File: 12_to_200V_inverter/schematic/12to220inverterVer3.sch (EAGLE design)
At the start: 246 parts, among them IC1 UC3842, IC10 TL494, IC2 PC817, IC3 LM358SOIC8, IC4 TL431, IC5 LM317, IC6 74HC595, IC7 74HC595, IC8 ATTINY45, T1 AO4407AL, T10 16N60, T11 BC847, T12 BC847, T13 BSS84, T14 BC857, T15 BC847, T16 BSS84, T17 BC847, T18 BC847, T19 BSS84, T2 IRF830, T20 BSS84, T21 BC847, T22 BC847, T23 BSS84, T24 BC847, T3 IRF830, T4 BC847, T5 BC857, T6 BC857, T7 IRFZ24N, T8 IRFZ24N, T9 BC857, X1 BAT+, X2 LAMP1, X3 LAMP1, X4 BAT-, X5 220VAC, X6 LAMP1_SWITCH, X7 LAMP1_SWITCH, X8 MCU_PROGRAMMING

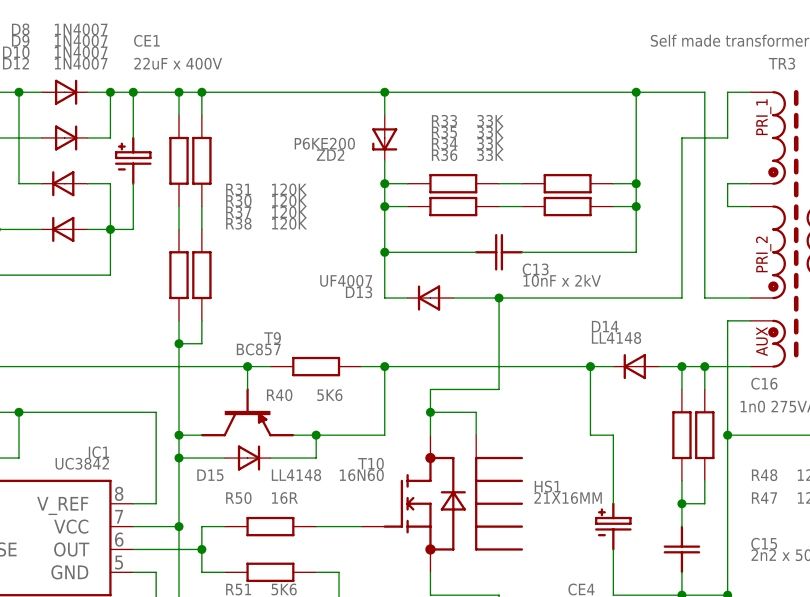
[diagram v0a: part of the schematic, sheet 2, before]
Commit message: 12 to 200V converter. Ver3. Start simplification.
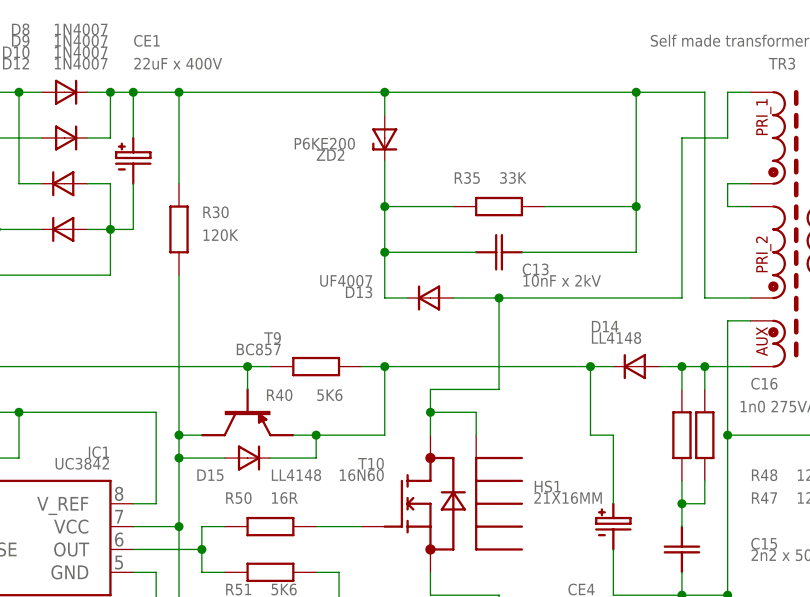
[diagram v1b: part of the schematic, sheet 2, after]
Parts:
- removed R31, R37, R38: 120K, __MyCommonLib1:RSMD_1206
- removed R33, R34, R36: 33K, __MyCommonLib1:RSMD_1206
- D10, D12, D13, D8, D9: device __MyCommonLib1:1N4001DO-41_5MM -> __MyCommonLib1:1N4001DO-41_10MM
- R30: device __MyCommonLib1:RSMD_1206 -> __MyCommonLib1:R1.0W
- R35: device __MyCommonLib1:RSMD_1206 -> __MyCommonLib1:R1.0W_VERT
- ZD2: device __MyCommonLib1:ZENNERDO-41_5MM -> __MyCommonLib1:ZENNERDO-41_10MM
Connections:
- removed net N$40: R31.PIN0, R38.PIN1
- removed net N$41: R30.PIN0, R37.PIN1
- removed net N$52: R33.PIN1, R34.PIN0
- removed net N$53: R35.PIN1, R36.PIN0
- net N$32: now also R35.PIN1; no longer R31.PIN1, R34.PIN1, R36.PIN1
- net N$36: no longer R33.PIN0
- net N$38: now also R30.PIN0; no longer R37.PIN0, R38.PIN0
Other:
- moved on the sheet: R30, R35
